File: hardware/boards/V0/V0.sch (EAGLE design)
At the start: 149 parts, among them IC2 TPS6300, J12 3.5mm TRRS Jack, J2 HIROSE_DM3BT-DSF-PEJSHIROSE_D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, J3 MOLEX_105450-0101MOLEX_105450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, Q2 ON_SEMI_MMBT5551LT1GON_SEMI_M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, U1 VS1053-L, U2 MICROCHIP_MCP73831T-2ATI-OTMI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, X3 FH12-45S-0.5SH

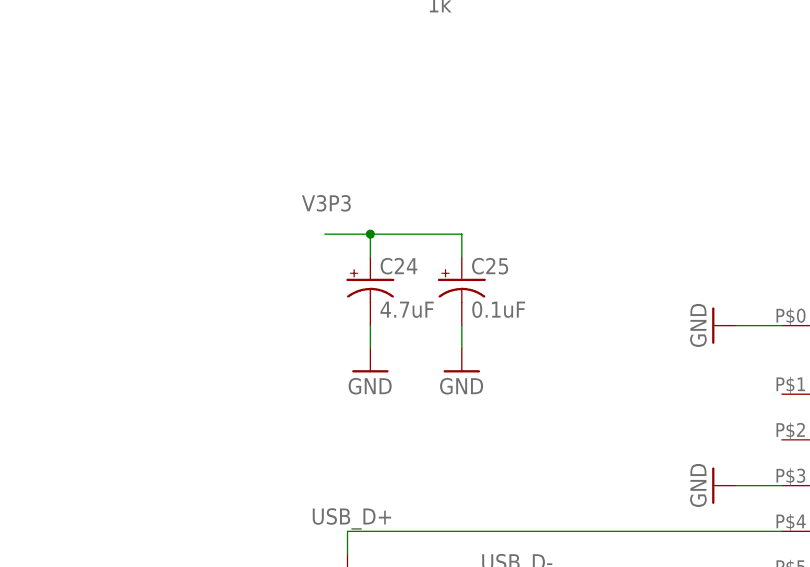
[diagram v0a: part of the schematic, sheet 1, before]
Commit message: checkpoint
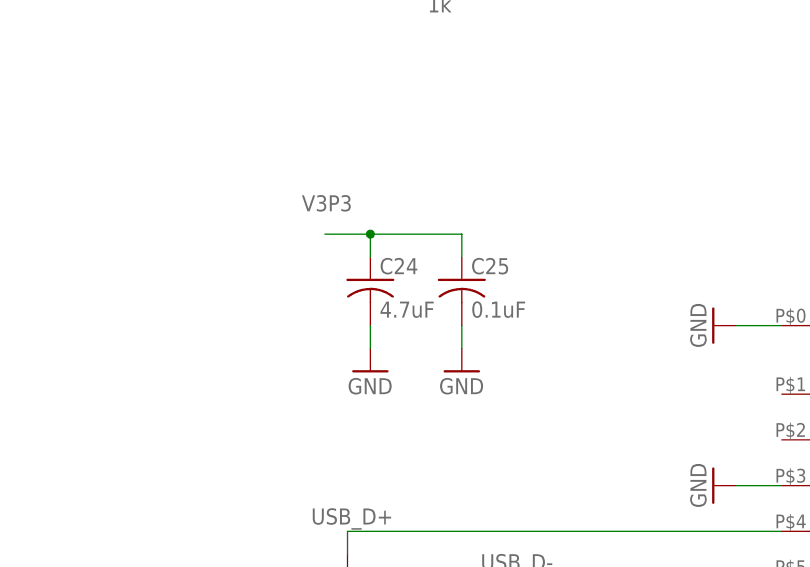
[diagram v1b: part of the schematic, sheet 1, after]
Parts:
- C24, C25: device rcl:CPOL-USC/6032-28R -> rcl:C-USC0402
- C34: device rcl:C-USC1206 -> rcl:C-USC0402
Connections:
- net GND: now also C24.2, C25.2; no longer C24.-, C25.-
- net V3P3: now also C24.1, C25.1; no longer C24.+, C25.+
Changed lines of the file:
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@@
 <?xml version="1.0" encoding="utf-8"?>
 <!DOCTYPE eagle SYSTEM "eagle.dtd">
-<eagle version="9.3.0">
+<eagle version="9.4.0">
 <drawing>
 <settings>
@@
 <part name="GND20" library="supply1" library_urn="urn:adsk.eagle:library:371" deviceset="GND" device=""/>
 <part name="GND23" library="supply1" library_urn="urn:adsk.eagle:library:371" deviceset="GND" device=""/>
-<part name="C24" library="rcl" library_urn="urn:adsk.eagle:library:334" deviceset="CPOL-US" device="C/6032-28R" package3d_urn="urn:adsk.eagle:package:23415/2" value="4.7uF"/>
-<part name="C25" library="rcl" library_urn="urn:adsk.eagle:library:334" deviceset="CPOL-US" device="C/6032-28R" package3d_urn="urn:adsk.eagle:package:23415/2" value="0.1uF"/>
+<part name="C24" library="rcl" library_urn="urn:adsk.eagle:library:334" deviceset="C-US" device="C0402" package3d_urn="urn:adsk.eagle:package:23626/2" value="4.7uF"/>
+<part name="C25" library="rcl" library_urn="urn:adsk.eagle:library:334" deviceset="C-US" device="C0402" package3d_urn="urn:adsk.eagle:package:23626/2" value="0.1uF"/>
 <part name="GND24" library="supply1" library_urn="urn:adsk.eagle:library:371" deviceset="GND" device=""/>
 <part name="GND25" library="supply1" library_urn="urn:adsk.eagle:library:371" deviceset="GND" device=""/>
@@
 <part name="GND43" library="supply1" library_urn="urn:adsk.eagle:library:371" deviceset="GND" device=""/>
 <part name="R50" library="rcl" library_urn="urn:adsk.eagle:library:334" deviceset="R-US_" device="R0402" package3d_urn="urn:adsk.eagle:package:23547/3" value="10k"/>
-<part name="C34" library="rcl" library_urn="urn:adsk.eagle:library:334" deviceset="C-US" device="C1206" package3d_urn="urn:adsk.eagle:package:23618/2" value="0.1uF"/>
+<part name="C34" library="rcl" library_urn="urn:adsk.eagle:library:334" deviceset="C-US" device="C0402" package3d_urn="urn:adsk.eagle:package:23626/2" value="0.1uF"/>
 <part name="GND44" library="supply1" library_urn="urn:adsk.eagle:library:371" deviceset="GND" device=""/>
 <part name="GND45" library="supply1" library_urn="urn:adsk.eagle:library:371" deviceset="GND" device=""/>
@@
 </segment>
 <segment>
-<pinref part="C24" gate="G$1" pin="-"/>
+<pinref part="C24" gate="G$1" pin="2"/>
 <wire x1="-182.88" y1="20.32" x2="-182.88" y2="17.78" width="0.1524" layer="91"/>
 <pinref part="GND24" gate="1" pin="GND"/>
 </segment>
 <segment>
-<pinref part="C25" gate="G$1" pin="-"/>
+<pinref part="C25" gate="G$1" pin="2"/>
 <wire x1="-172.72" y1="20.32" x2="-172.72" y2="17.78" width="0.1524" layer="91"/>
 <pinref part="GND25" gate="1" pin="GND"/>
@@
 </segment>
 <segment>
-<pinref part="C25" gate="G$1" pin="+"/>
+<pinref part="C25" gate="G$1" pin="1"/>
 <wire x1="-172.72" y1="30.48" x2="-172.72" y2="27.94" width="0.1524" layer="91"/>
-<pinref part="C24" gate="G$1" pin="+"/>
+<pinref part="C24" gate="G$1" pin="1"/>
 <wire x1="-182.88" y1="27.94" x2="-182.88" y2="30.48" width="0.1524" layer="91"/>
 <label x="-190.5" y="33.02" size="1.778" layer="95"/>
@@
 packages will not be understood (or retained) with this version.
 </note>
-<note version="8.4" severity="warning">
-Since Version 8.4, EAGLE supports properties for SPICE simulation.
-Probes in schematics and SPICE mapping objects found in parts and library devices
-will not be understood with this version. Update EAGLE to the latest version
-for full support of SPICE simulation.
-</note>
 </compatibility>
